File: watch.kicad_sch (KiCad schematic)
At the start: 74 parts, among them U1 DS3231MZ_TRL, U2 ATMEGA328P-AU

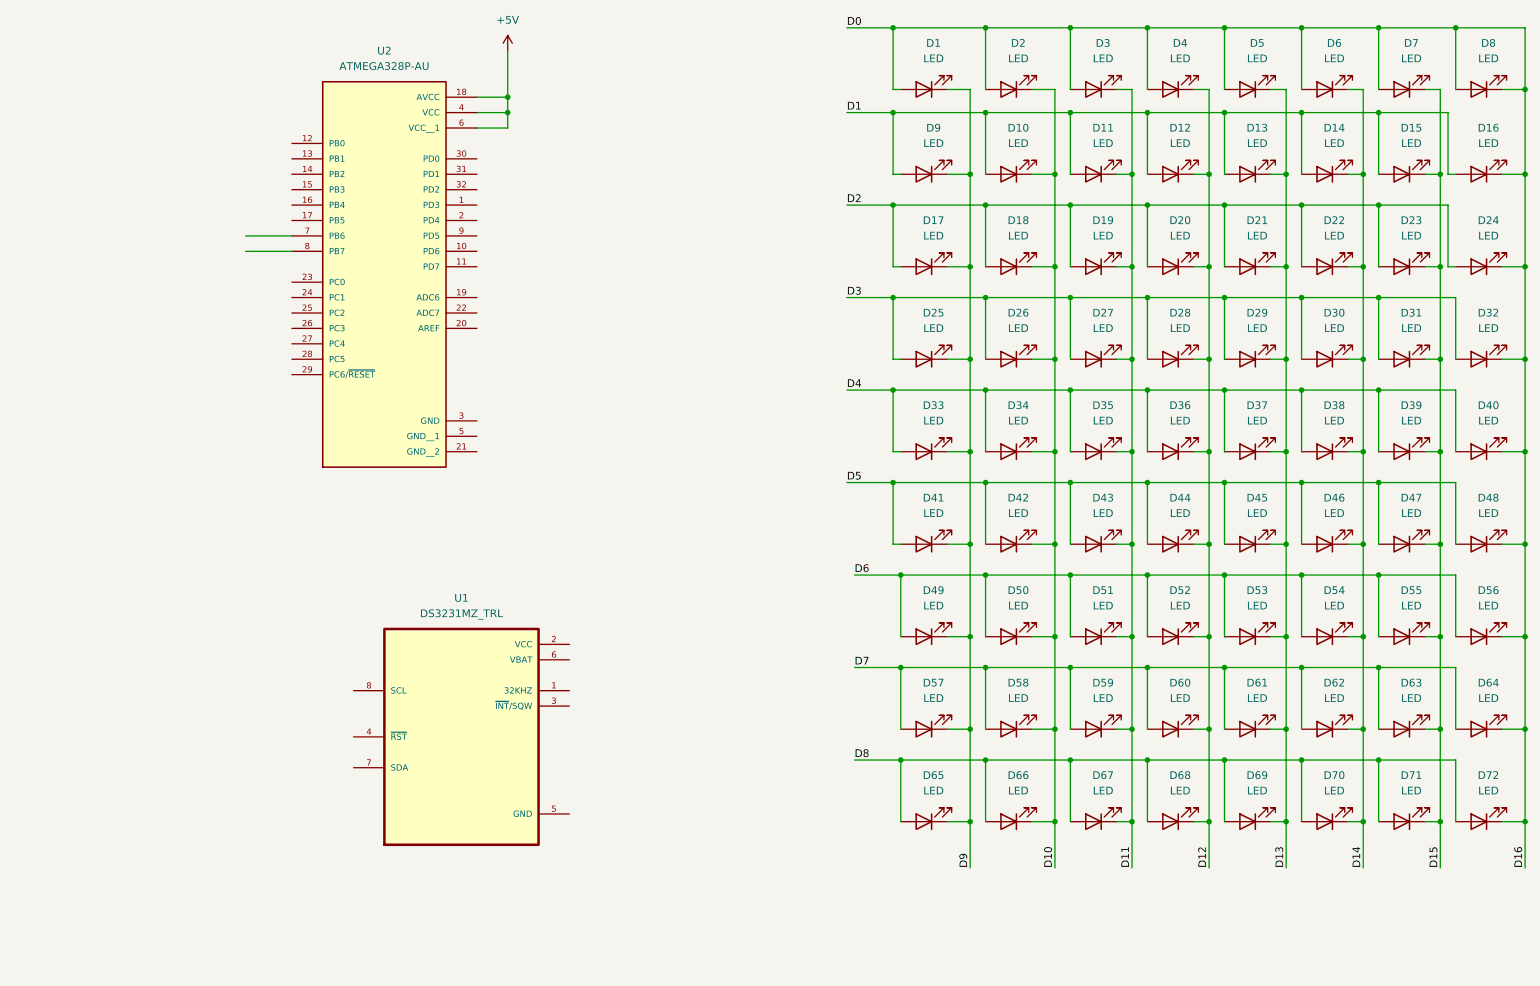
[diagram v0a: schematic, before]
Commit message: :D
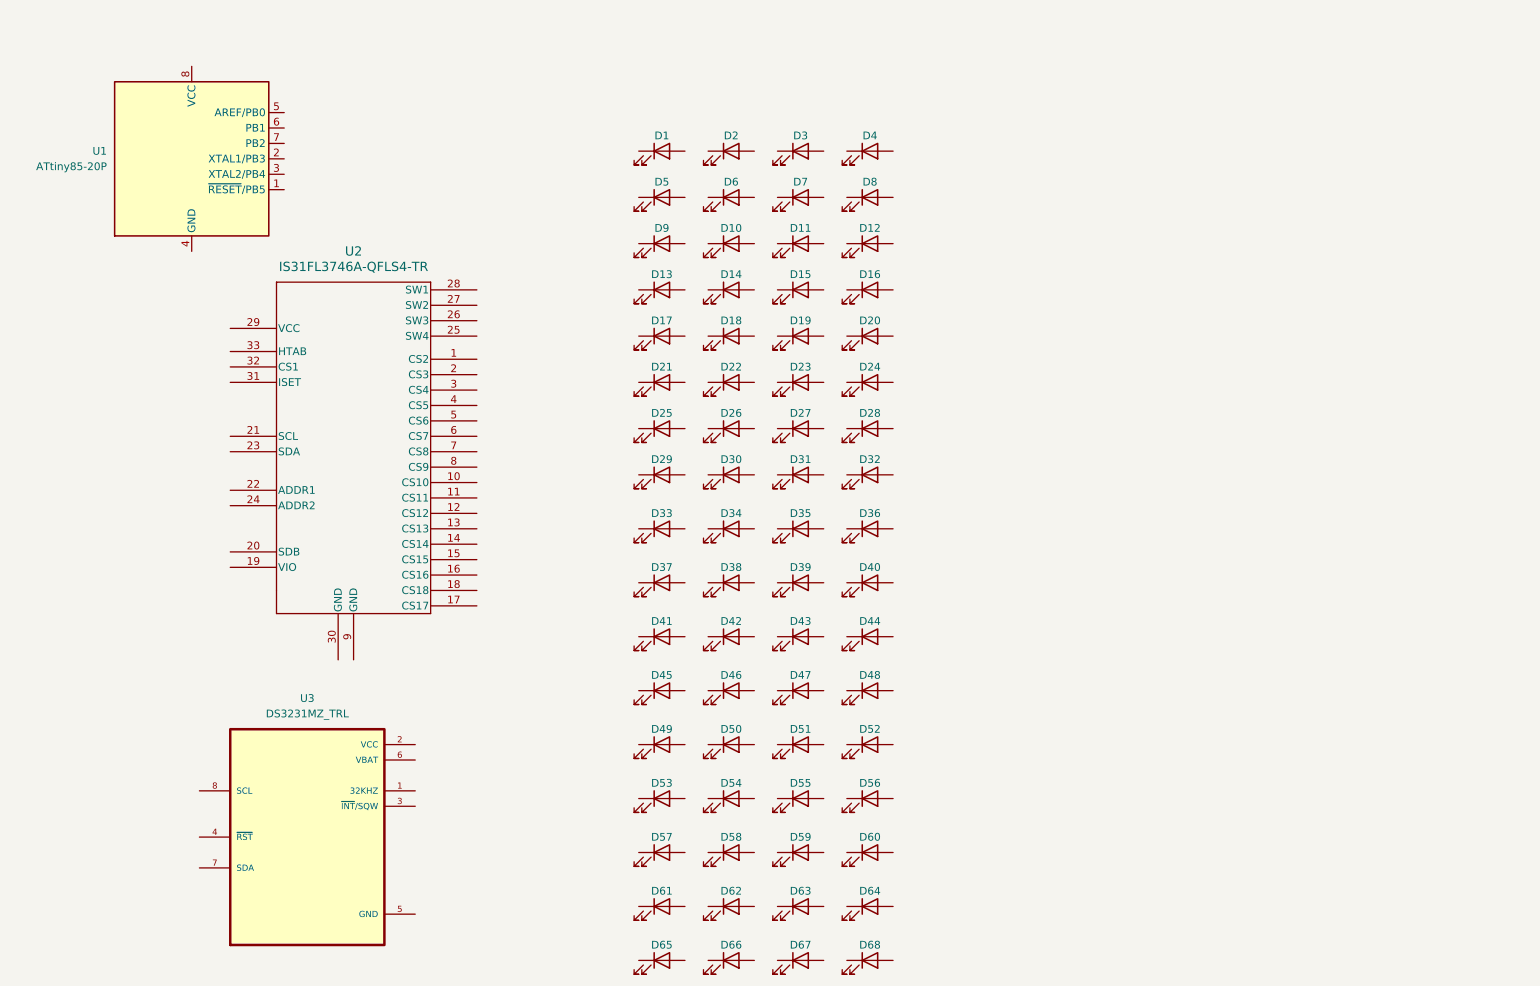
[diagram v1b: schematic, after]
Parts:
- removed D69, D70, D71, D72: LED, symbol Device:LED
- removed U2: ATMEGA328P-AU, ATMEGA328P-AU:QFP80P900X900X120-32N, symbol ESC:ATMEGA328P-AU
- added U1: ATtiny85-20P, Package_DIP:DIP-8_W7.62mm, symbol MCU_Microchip_ATtiny:ATtiny85-20P
- added U2: IS31FL3746A-QFLS4-TR, QFN-32_ISI, symbol ESC:IS31FL3746A-QFLS4-TR
- D1, D10, D11, D12, D13, D14, D15, D16, D17, D18, D19, D2, D20, D21, D22, D23, D24, D25, D26, D27, D28, D29, D3, D30, D31, D32, D33, D34, D35, D36, D37, D38, D39, D4, D40, D41, D42, D43, D44, D45, D46, D47, D48, D49, D5, D50, D51, D52, D53, D54, D55, D56, D57, D58, D59, D6, D60, D61, D62, D63, D64, D65, D66, D67, D68, D7, D8, D9: value LED -> ~
- renumbered U1 to U3
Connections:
- removed net D0: D1.2 (A), D16.1 (K), D2.2 (A), D24.1 (K), D3.2 (A), D32.1 (K), D4.2 (A), D40.1 (K), D48.1 (K), D5.2 (A), D56.1 (K), D6.2 (A), D64.1 (K), D7.2 (A), D8.1 (K), D8.2 (A)
- removed net D1: D10.2 (A), D11.2 (A), D12.2 (A), D13.2 (A), D14.2 (A), D15.2 (A), D16.2 (A), D9.2 (A)
- removed net D10: D10.1 (K), D18.1 (K), D2.1 (K), D26.1 (K), D34.1 (K), D42.1 (K), D50.1 (K), D58.1 (K), D66.1 (K)
- removed net D11: D11.1 (K), D19.1 (K), D27.1 (K), D3.1 (K), D35.1 (K), D43.1 (K), D51.1 (K), D59.1 (K), D67.1 (K)
- removed net D12: D12.1 (K), D20.1 (K), D28.1 (K), D36.1 (K), D4.1 (K), D44.1 (K), D52.1 (K), D60.1 (K), D68.1 (K)
- removed net D13: D13.1 (K), D21.1 (K), D29.1 (K), D37.1 (K), D45.1 (K), D5.1 (K), D53.1 (K), D61.1 (K)
- removed net D14: D14.1 (K), D22.1 (K), D30.1 (K), D38.1 (K), D46.1 (K), D54.1 (K), D6.1 (K), D62.1 (K)
- removed net D15: D15.1 (K), D23.1 (K), D31.1 (K), D39.1 (K), D47.1 (K), D55.1 (K), D63.1 (K), D7.1 (K)
- removed net D2: D17.2 (A), D18.2 (A), D19.2 (A), D20.2 (A), D21.2 (A), D22.2 (A), D23.2 (A), D24.2 (A)
- removed net D3: D25.2 (A), D26.2 (A), D27.2 (A), D28.2 (A), D29.2 (A), D30.2 (A), D31.2 (A), D32.2 (A)
- removed net D4: D33.2 (A), D34.2 (A), D35.2 (A), D36.2 (A), D37.2 (A), D38.2 (A), D39.2 (A), D40.2 (A)
- removed net D5: D41.2 (A), D42.2 (A), D43.2 (A), D44.2 (A), D45.2 (A), D46.2 (A), D47.2 (A), D48.2 (A)
- removed net D6: D49.2 (A), D50.2 (A), D51.2 (A), D52.2 (A), D53.2 (A), D54.2 (A), D55.2 (A), D56.2 (A)
- removed net D7: D57.2 (A), D58.2 (A), D59.2 (A), D60.2 (A), D61.2 (A), D62.2 (A), D63.2 (A), D64.2 (A)
- removed net D8: D65.2 (A), D66.2 (A), D67.2 (A), D68.2 (A)
- removed net D9: D1.1 (K), D17.1 (K), D25.1 (K), D33.1 (K), D41.1 (K), D49.1 (K), D57.1 (K), D65.1 (K), D9.1 (K)
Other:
- moved on the sheet: U3
